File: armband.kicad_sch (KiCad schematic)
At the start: 33 parts, among them IC1 STM32MP157AAB3, IC7 S40FC004C1B2C00000, IC9 NXS0506UPZ, J3 MEM2075-00-140-01-A, J4 Conn_01x03, SW1 SW_MEC_5G, SW2 SW_MEC_5G

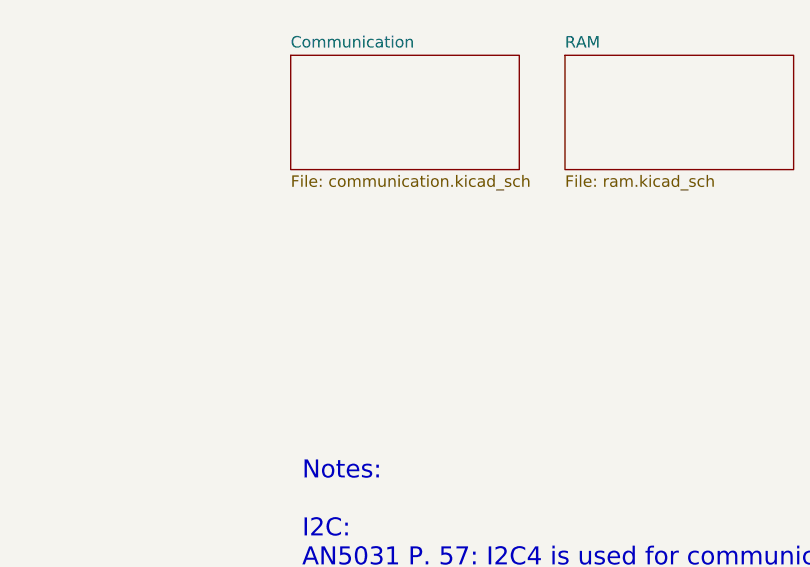
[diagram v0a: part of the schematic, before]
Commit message: added flash
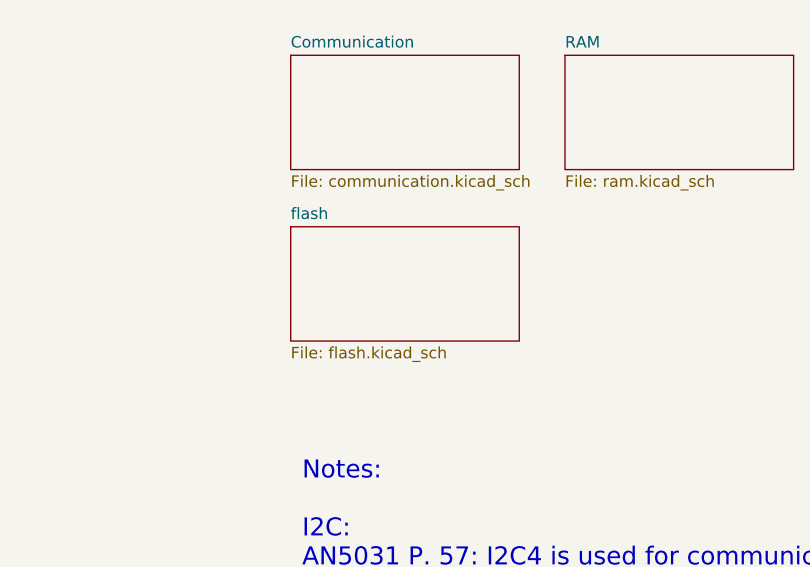
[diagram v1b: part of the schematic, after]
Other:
- added sheet flash (flash.kicad_sch)
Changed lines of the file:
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@@
+    )
+  )
+  (sheet (at 299.72 222.25) (size 25.4 12.7) (fields_autoplaced)
+    (stroke (width 0.1524) (type solid))
+    (fill (color 0 0 0 0.0000))
+    (property "Sheetname" "flash" (at 299.72 221.5384 0)
+      (effects (font (size 1.27 1.27)) (justify left bottom))
+    )
+    (property "Sheetfile" "flash.kicad_sch" (at 299.72 235.5346 0)
+      (effects (font (size 1.27 1.27)) (justify left top))
+    )
+    (instances
+      (project "armband"
+        (path "/017c50c6-333c-4d31-ad5a-278994a09b14" (page "5"))
+      )
     )
   )
